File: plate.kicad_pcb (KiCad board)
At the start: 2 copper layers, 146.8 x 120.4 mm, 0 parts

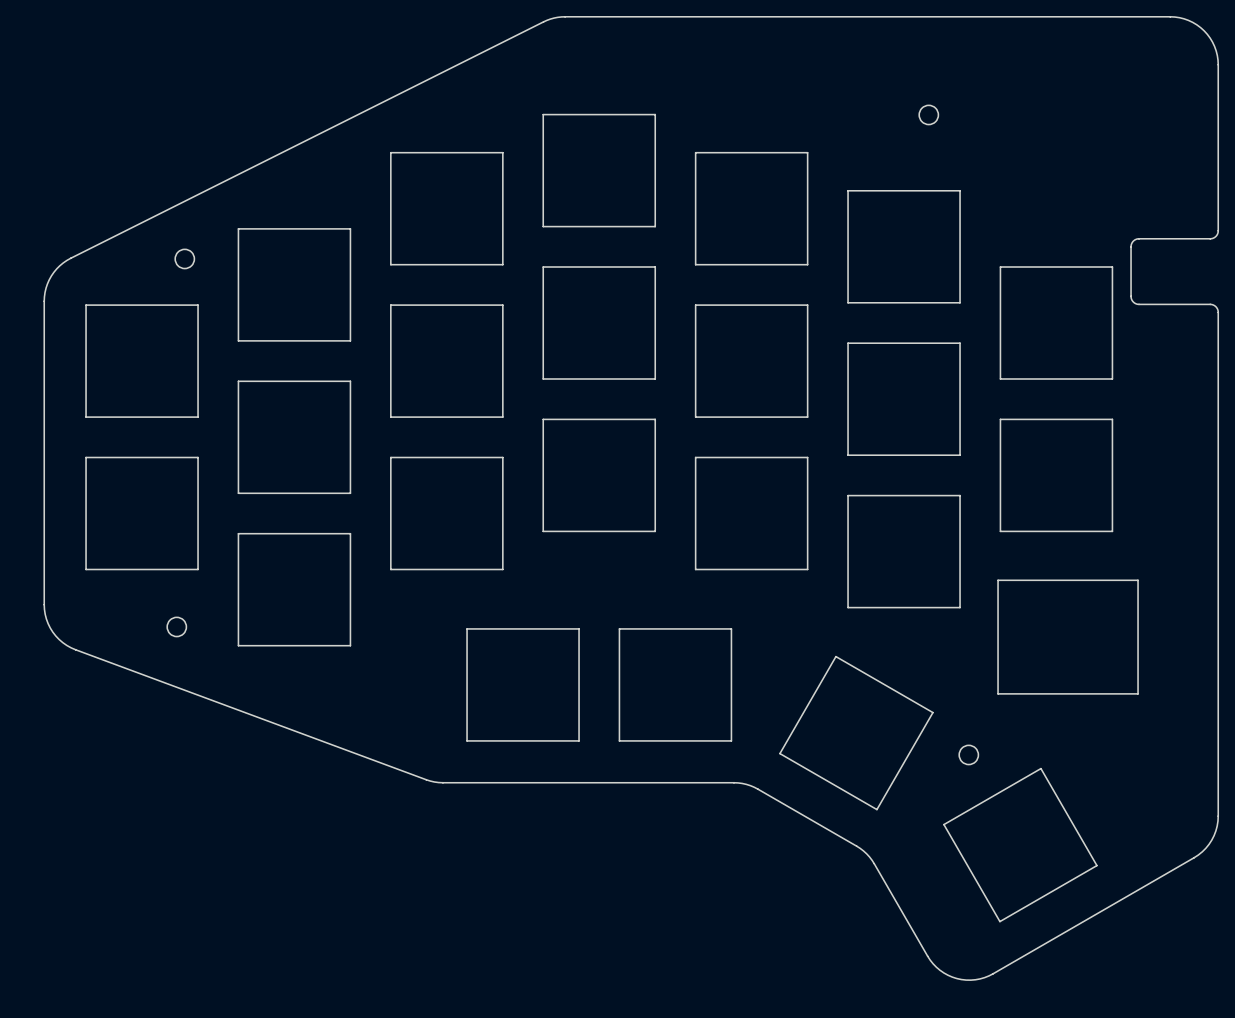
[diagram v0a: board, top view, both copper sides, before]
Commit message: :sparkles: (all) ready for manufacturing
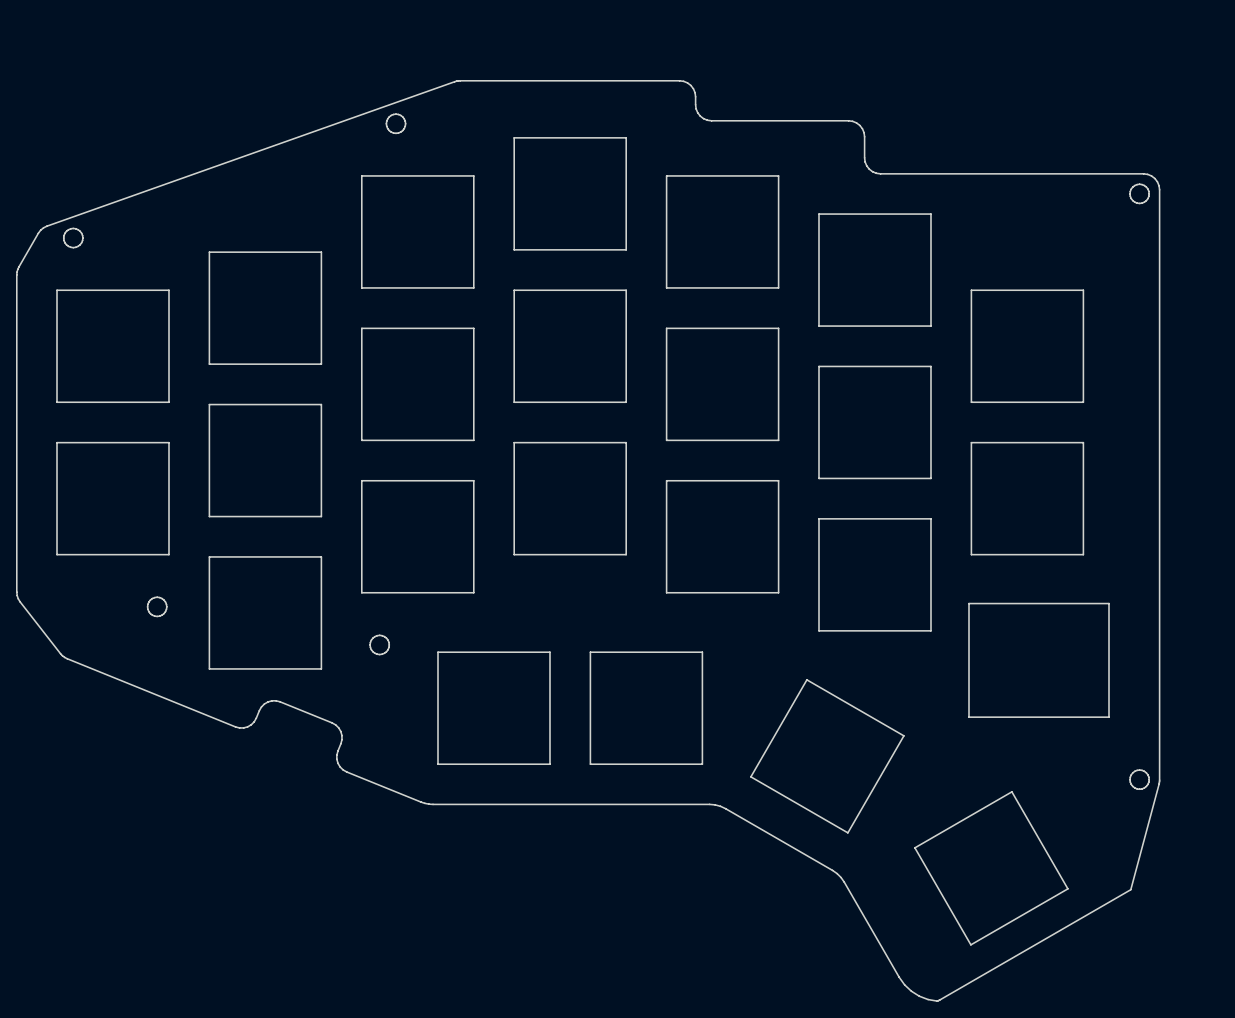
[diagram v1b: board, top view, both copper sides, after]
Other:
- board size 146.8 x 120.4 mm -> 142.8 x 115 mm
